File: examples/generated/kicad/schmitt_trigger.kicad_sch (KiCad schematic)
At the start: 6 parts

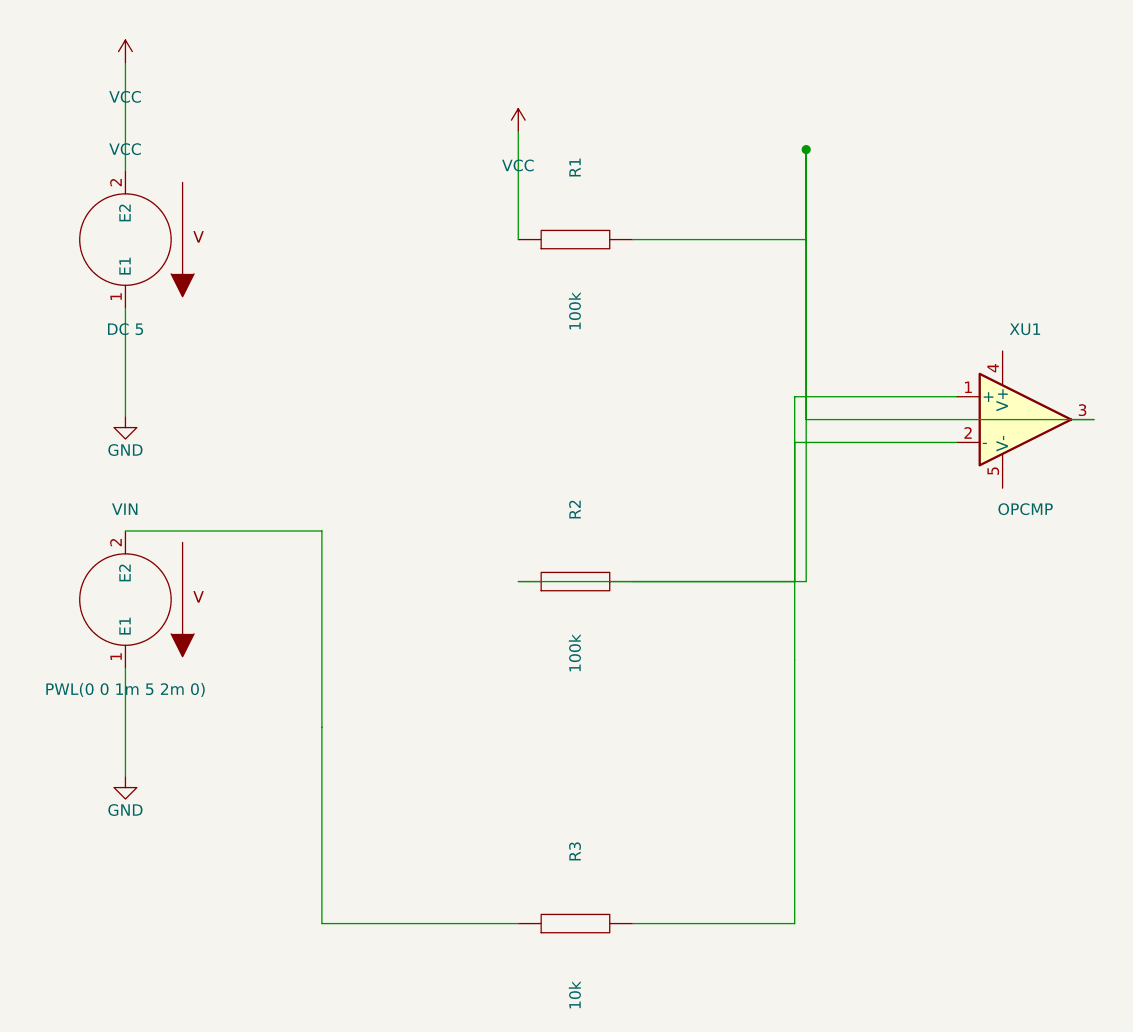
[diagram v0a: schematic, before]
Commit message: Attempt to correct strange wiring.
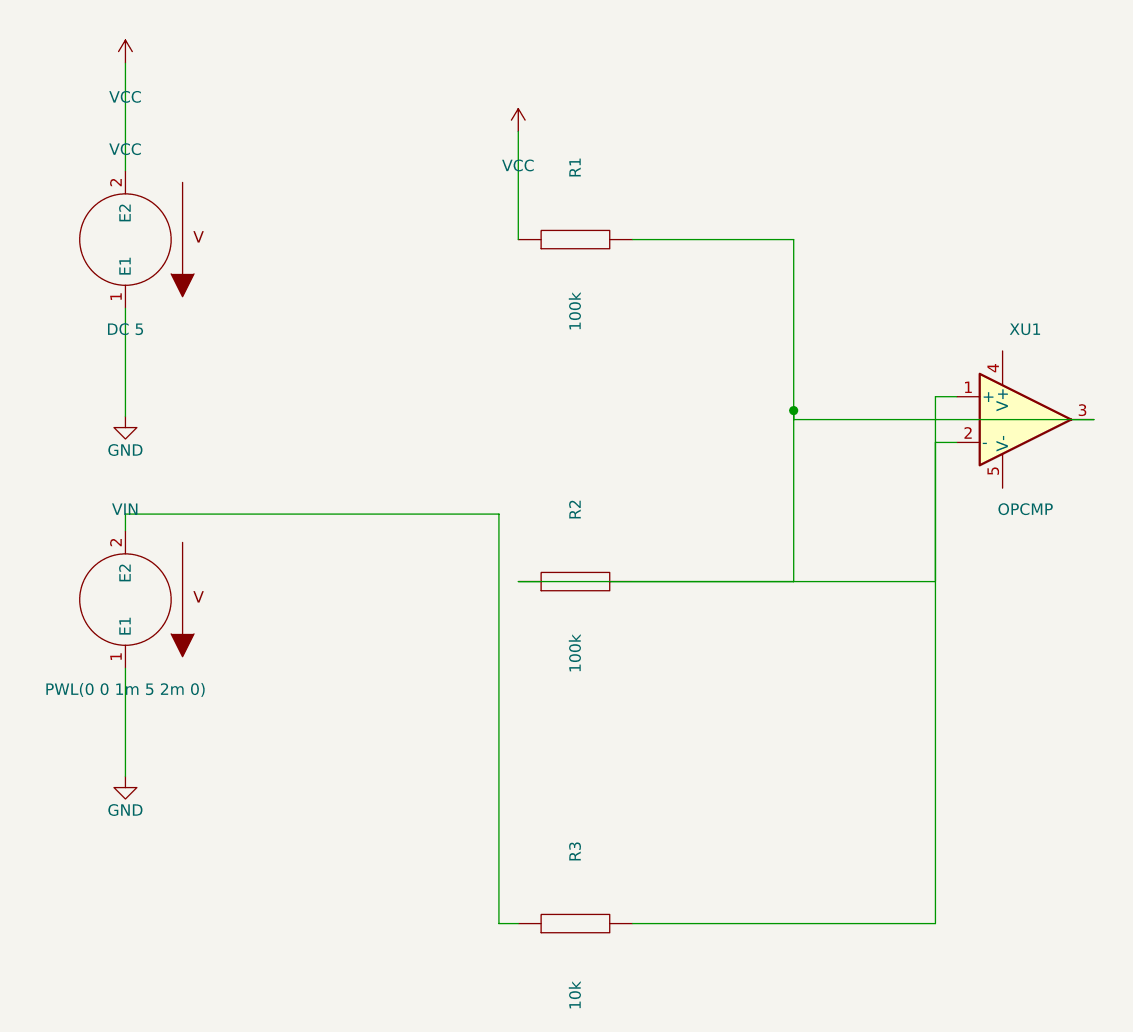
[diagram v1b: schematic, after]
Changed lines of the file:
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@@
     (stroke (width 0) (type solid) (color 0 0 0 0))
   )
-  (wire (pts (xy 50.00 102.38) (xy 71.83 102.38))
+  (wire (pts (xy 50.00 102.38) (xy 50.00 100.50))
     (stroke (width 0) (type solid) (color 0 0 0 0))
   )
-  (wire (pts (xy 71.83 102.38) (xy 71.83 124.19))
+  (wire (pts (xy 50.00 100.50) (xy 91.50 100.50))
     (stroke (width 0) (type solid) (color 0 0 0 0))
   )
-  (wire (pts (xy 93.65 146.00) (xy 71.83 146.00))
+  (wire (pts (xy 91.50 100.50) (xy 91.50 146.00))
     (stroke (width 0) (type solid) (color 0 0 0 0))
   )
-  (wire (pts (xy 71.83 146.00) (xy 71.83 124.19))
+  (wire (pts (xy 91.50 146.00) (xy 93.65 146.00))
     (stroke (width 0) (type solid) (color 0 0 0 0))
   )
-  (wire (pts (xy 106.35 146.00) (xy 124.36 146.00))
+  (wire (pts (xy 106.35 146.00) (xy 140.00 146.00))
     (stroke (width 0) (type solid) (color 0 0 0 0))
   )
-  (wire (pts (xy 124.36 146.00) (xy 124.36 116.73))
+  (wire (pts (xy 140.00 146.00) (xy 140.00 87.46))
     (stroke (width 0) (type solid) (color 0 0 0 0))
   )
-  (wire (pts (xy 142.38 87.46) (xy 124.36 87.46))
+  (wire (pts (xy 140.00 87.46) (xy 142.38 87.46))
     (stroke (width 0) (type solid) (color 0 0 0 0))
   )
-  (wire (pts (xy 124.36 87.46) (xy 124.36 116.73))
+  (wire (pts (xy 106.35 70.00) (xy 124.25 70.00))
     (stroke (width 0) (type solid) (color 0 0 0 0))
   )
-  (wire (pts (xy 106.35 70.00) (xy 125.64 70.00))
+  (wire (pts (xy 124.25 70.00) (xy 124.25 89.00))
     (stroke (width 0) (type solid) (color 0 0 0 0))
   )
-  (wire (pts (xy 125.64 70.00) (xy 125.64 60.00))
+  (wire (pts (xy 93.65 108.00) (xy 124.25 108.00))
     (stroke (width 0) (type solid) (color 0 0 0 0))
   )
-  (wire (pts (xy 93.65 108.00) (xy 125.64 108.00))
+  (wire (pts (xy 124.25 108.00) (xy 124.25 89.00))
     (stroke (width 0) (type solid) (color 0 0 0 0))
   )
-  (wire (pts (xy 125.64 108.00) (xy 125.64 60.00))
+  (wire (pts (xy 157.62 90.00) (xy 124.25 90.00))
     (stroke (width 0) (type solid) (color 0 0 0 0))
   )
-  (wire (pts (xy 157.62 90.00) (xy 125.64 90.00))
+  (wire (pts (xy 124.25 90.00) (xy 124.25 89.00))
     (stroke (width 0) (type solid) (color 0 0 0 0))
   )
-  (wire (pts (xy 125.64 90.00) (xy 125.64 60.00))
+  (wire (pts (xy 106.35 108.00) (xy 140.00 108.00))
     (stroke (width 0) (type solid) (color 0 0 0 0))
   )
-  (wire (pts (xy 106.35 108.00) (xy 124.36 108.00))
+  (wire (pts (xy 140.00 108.00) (xy 140.00 92.54))
     (stroke (width 0) (type solid) (color 0 0 0 0))
   )
-  (wire (pts (xy 124.36 108.00) (xy 124.36 100.27))
+  (wire (pts (xy 140.00 92.54) (xy 142.38 92.54))
     (stroke (width 0) (type solid) (color 0 0 0 0))
   )
-  (wire (pts (xy 142.38 92.54) (xy 124.36 92.54))
-    (stroke (width 0) (type solid) (color 0 0 0 0))
-  )
-  (wire (pts (xy 124.36 92.54) (xy 124.36 100.27))
-    (stroke (width 0) (type solid) (color 0 0 0 0))
-  )
-  (junction (at 125.64 60.00) (diameter 1.016) (color 0 0 0 0))
+  (junction (at 124.25 89.00) (diameter 1.016) (color 0 0 0 0))
   (sheet_instances
     (path "/" (page "1"))

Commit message: Attempt shape and wiring fixes again.
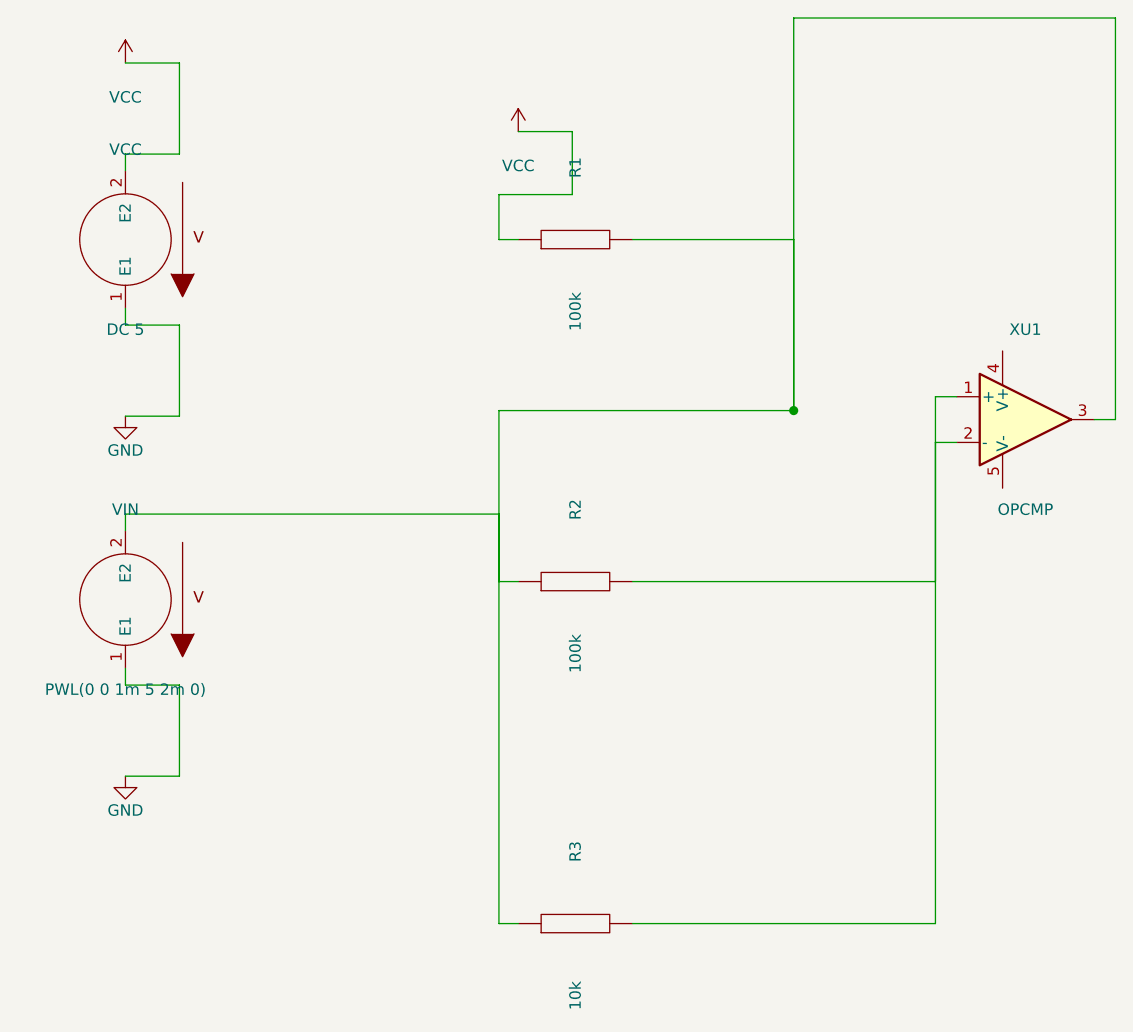
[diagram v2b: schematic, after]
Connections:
- net at R3.1, VIN.2 (E2): now also R1.2, R2.1, XU1.3
- net at R2.2, R3.2, XU1.1 (+)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: no longer R1.2, R2.1, XU1.3
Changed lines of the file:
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@@
     )
   )
-  (wire (pts (xy 50.00 62.38) (xy 50.00 50.38))
+  (wire (pts (xy 50.00 62.38) (xy 50.00 60.50))
     (stroke (width 0) (type solid) (color 0 0 0 0))
   )
-  (wire (pts (xy 50.00 77.62) (xy 50.00 89.62))
+  (wire (pts (xy 50.00 60.50) (xy 56.00 60.50))
     (stroke (width 0) (type solid) (color 0 0 0 0))
   )
-  (wire (pts (xy 50.00 117.62) (xy 50.00 129.62))
+  (wire (pts (xy 56.00 60.50) (xy 56.00 50.38))
     (stroke (width 0) (type solid) (color 0 0 0 0))
   )
-  (wire (pts (xy 93.65 70.00) (xy 93.65 58.00))
+  (wire (pts (xy 56.00 50.38) (xy 50.00 50.38))
+    (stroke (width 0) (type solid) (color 0 0 0 0))
+  )
+  (wire (pts (xy 50.00 77.62) (xy 50.00 79.50))
+    (stroke (width 0) (type solid) (color 0 0 0 0))
+  )
+  (wire (pts (xy 50.00 79.50) (xy 56.00 79.50))
+    (stroke (width 0) (type solid) (color 0 0 0 0))
+  )
+  (wire (pts (xy 56.00 79.50) (xy 56.00 89.62))
+    (stroke (width 0) (type solid) (color 0 0 0 0))
+  )
+  (wire (pts (xy 56.00 89.62) (xy 50.00 89.62))
+    (stroke (width 0) (type solid) (color 0 0 0 0))
+  )
+  (wire (pts (xy 50.00 117.62) (xy 50.00 119.50))
+    (stroke (width 0) (type solid) (color 0 0 0 0))
+  )
+  (wire (pts (xy 50.00 119.50) (xy 56.00 119.50))
+    (stroke (width 0) (type solid) (color 0 0 0 0))
+  )
+  (wire (pts (xy 56.00 119.50) (xy 56.00 129.62))
+    (stroke (width 0) (type solid) (color 0 0 0 0))
+  )
+  (wire (pts (xy 56.00 129.62) (xy 50.00 129.62))
+    (stroke (width 0) (type solid) (color 0 0 0 0))
+  )
+  (wire (pts (xy 93.65 70.00) (xy 91.50 70.00))
+    (stroke (width 0) (type solid) (color 0 0 0 0))
+  )
+  (wire (pts (xy 91.50 70.00) (xy 91.50 65.00))
+    (stroke (width 0) (type solid) (color 0 0 0 0))
+  )
+  (wire (pts (xy 91.50 65.00) (xy 99.65 65.00))
+    (stroke (width 0) (type solid) (color 0 0 0 0))
+  )
+  (wire (pts (xy 99.65 65.00) (xy 99.65 58.00))
+    (stroke (width 0) (type solid) (color 0 0 0 0))
+  )
+  (wire (pts (xy 99.65 58.00) (xy 93.65 58.00))
     (stroke (width 0) (type solid) (color 0 0 0 0))
   )
@@
     (stroke (width 0) (type solid) (color 0 0 0 0))
   )
-  (wire (pts (xy 93.65 108.00) (xy 124.25 108.00))
+  (wire (pts (xy 93.65 108.00) (xy 91.50 108.00))
     (stroke (width 0) (type solid) (color 0 0 0 0))
   )
-  (wire (pts (xy 124.25 108.00) (xy 124.25 89.00))
+  (wire (pts (xy 91.50 108.00) (xy 91.50 89.00))
     (stroke (width 0) (type solid) (color 0 0 0 0))
   )
-  (wire (pts (xy 157.62 90.00) (xy 124.25 90.00))
+  (wire (pts (xy 91.50 89.00) (xy 124.25 89.00))
     (stroke (width 0) (type solid) (color 0 0 0 0))
   )
-  (wire (pts (xy 124.25 90.00) (xy 124.25 89.00))
+  (wire (pts (xy 157.62 90.00) (xy 160.00 90.00))
     (stroke (width 0) (type solid) (color 0 0 0 0))
   )
+  (wire (pts (xy 160.00 90.00) (xy 160.00 45.38))
+    (stroke (width 0) (type solid) (color 0 0 0 0))
+  )
+  (wire (pts (xy 160.00 45.38) (xy 124.25 45.38))
+    (stroke (width 0) (type solid) (color 0 0 0 0))
+  )
+  (wire (pts (xy 124.25 45.38) (xy 124.25 89.00))
+    (stroke (width 0) (type solid) (color 0 0 0 0))
+  )
